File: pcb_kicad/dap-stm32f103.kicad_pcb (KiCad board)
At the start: 2 copper layers, 41.7 x 26.9 mm, 35 parts, among them J1 USB_C_Receptacle_USB2.0, U1 STM32F103CBTx, Y1 SMD-5032_2P_8MHz_20ppm_20pF

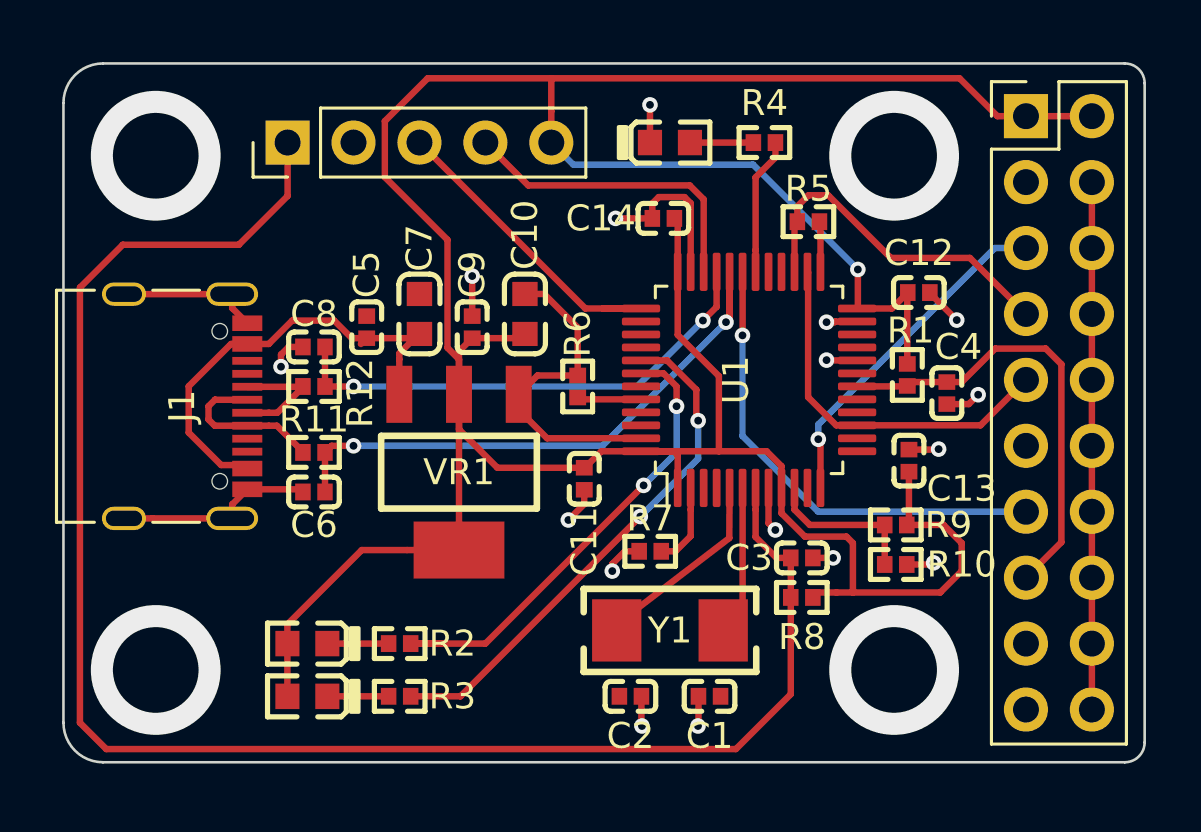
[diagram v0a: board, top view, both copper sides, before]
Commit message: [pcb] done
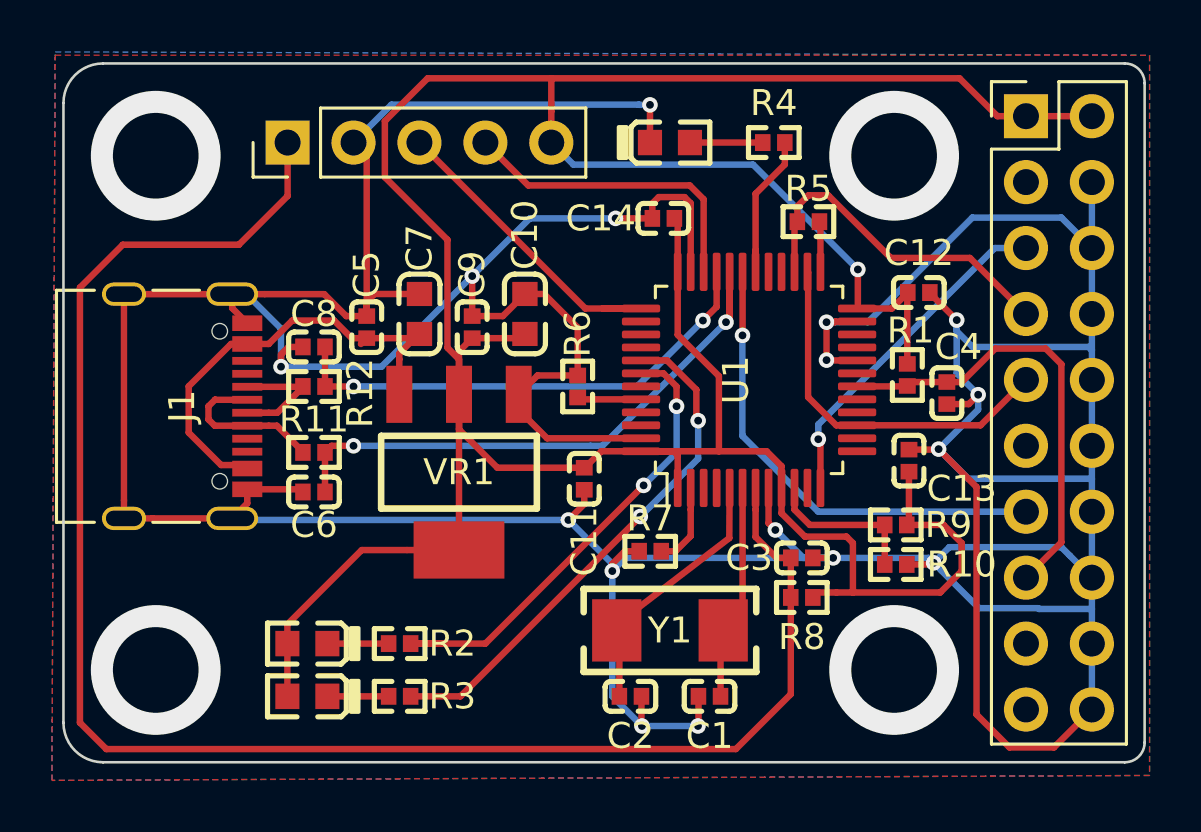
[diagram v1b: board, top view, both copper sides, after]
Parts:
- moved R4 0.36 mm to (145.7, 139.2)
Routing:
- net GND: track 72.2 -> 231.3 mm
- net Net-(C1-Pad2): track 5.80 -> 8.38 mm
- net Net-(C2-Pad2): track 7.63 -> 10.2 mm
- net /LED_RED: track 5.30 -> 6.29 mm
- added copper zone on B.Cu, net GND
- added copper zone on F.Cu, net GND
